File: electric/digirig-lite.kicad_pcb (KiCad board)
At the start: 2 copper layers, 16 x 37 mm, 54 parts, among them Q1 MMBT5551L, Q2 MMBT5551L, Q3 MMBT5551L, U1 CM108

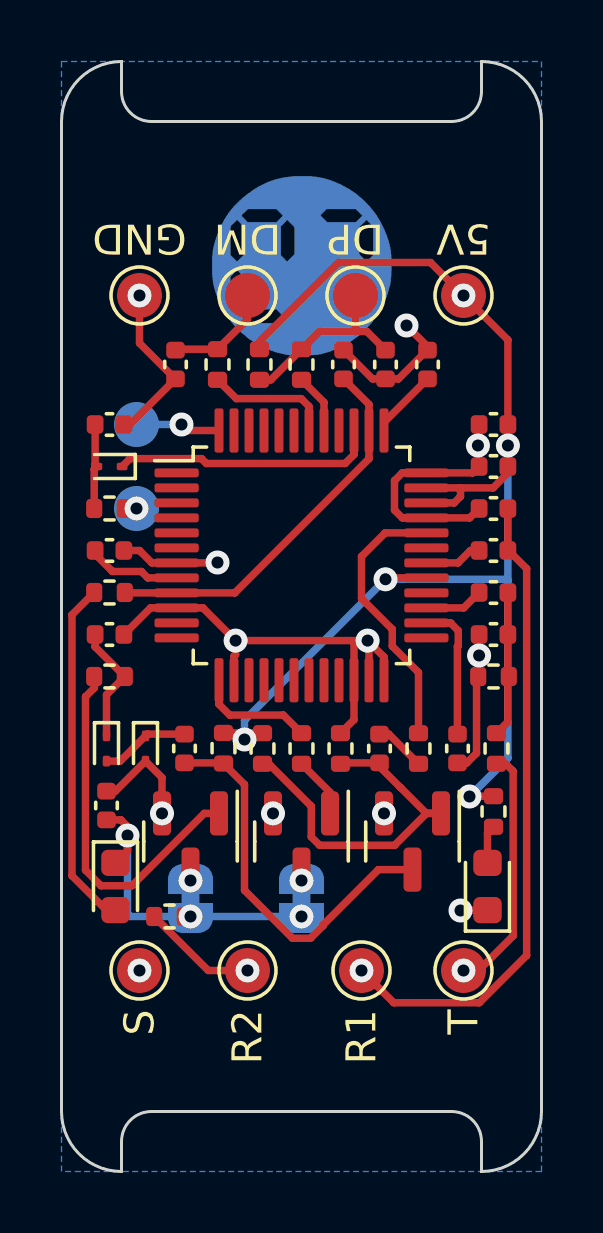
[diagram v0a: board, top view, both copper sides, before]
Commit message: Revision 1.2
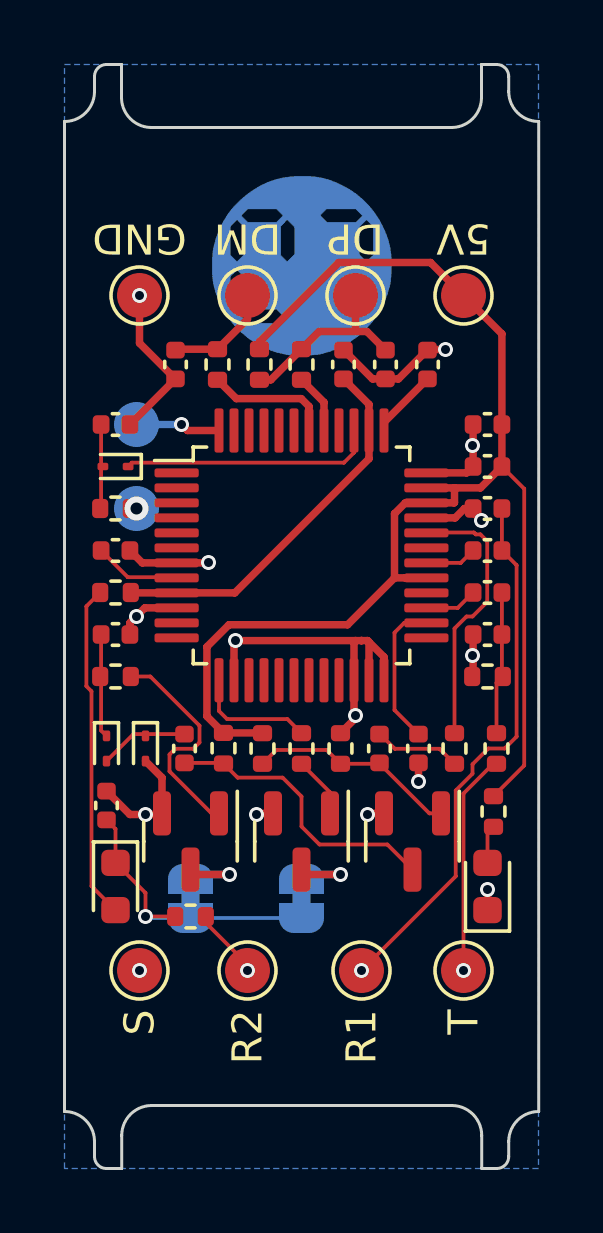
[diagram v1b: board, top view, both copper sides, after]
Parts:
- moved C7 1.30 mm to (140.4, 91.6)
- moved R5 1.20 mm to (141.7, 91.6)
- moved R14 0.70 mm to (132.8, 97.2), turned to 180 degrees
- moved C10 0.20 mm to (142.8, 85.0)
- moved C12 0.20 mm to (130.3, 80.8)
- moved C14 0.20 mm to (130.3, 87.8)
- moved C15 0.20 mm to (142.8, 87.8)
- moved C16 0.20 mm to (142.8, 83.6)
- moved C2 0.20 mm to (142.8, 80.8)
- moved C4 0.20 mm to (142.8, 82.2)
- moved C5 0.20 mm to (130.3, 85.0)
- moved C9 0.20 mm to (142.8, 86.4)
- moved D2 0.20 mm to (130.3, 82.2)
- moved R10 0.20 mm to (142.8, 89.2)
- moved R11 0.20 mm to (130.3, 89.2), turned to 180 degrees
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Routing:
- net GND: track 47.9 -> 39.9 mm, vias 12 -> 15
- net Net-(Q1-B): track 12.2 -> 7.05 mm
- net Net-(Q2-B): track 12.2 -> 7.49 mm
- net /RIG_AFIN: track 21.8 -> 18.1 mm
- net Net-(Q1-C): track 13.0 -> 9.66 mm
- net Net-(JP1-A): track 0.00 -> 2.73 mm
- net Net-(JP2-A): track 0.00 -> 2.73 mm
- net /RIG_PTT: track 3.86 -> 2.38 mm
- net Net-(C11-Pad2): track 1.71 -> 2.91 mm
- net /RIG_AFOUT: track 8.28 -> 7.41 mm
- net +5V: track 46.7 -> 47.5 mm, vias 5 -> 0
- net Net-(D5-K): track 10.7 -> 9.97 mm, vias 3 -> 1
- net Net-(D4-K): track 4.04 -> 3.45 mm
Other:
- board size 16 x 37 mm -> 15.8 x 36.8 mm
